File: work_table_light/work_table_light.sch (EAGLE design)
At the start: 38 parts, among them IC1 TINY24/44/84-PU, Q1 IRFP250, Q2 IRFP250, Q3 IRFP250, Q4 IRFP250, Q6 IRFP250, Q7 IRFP250

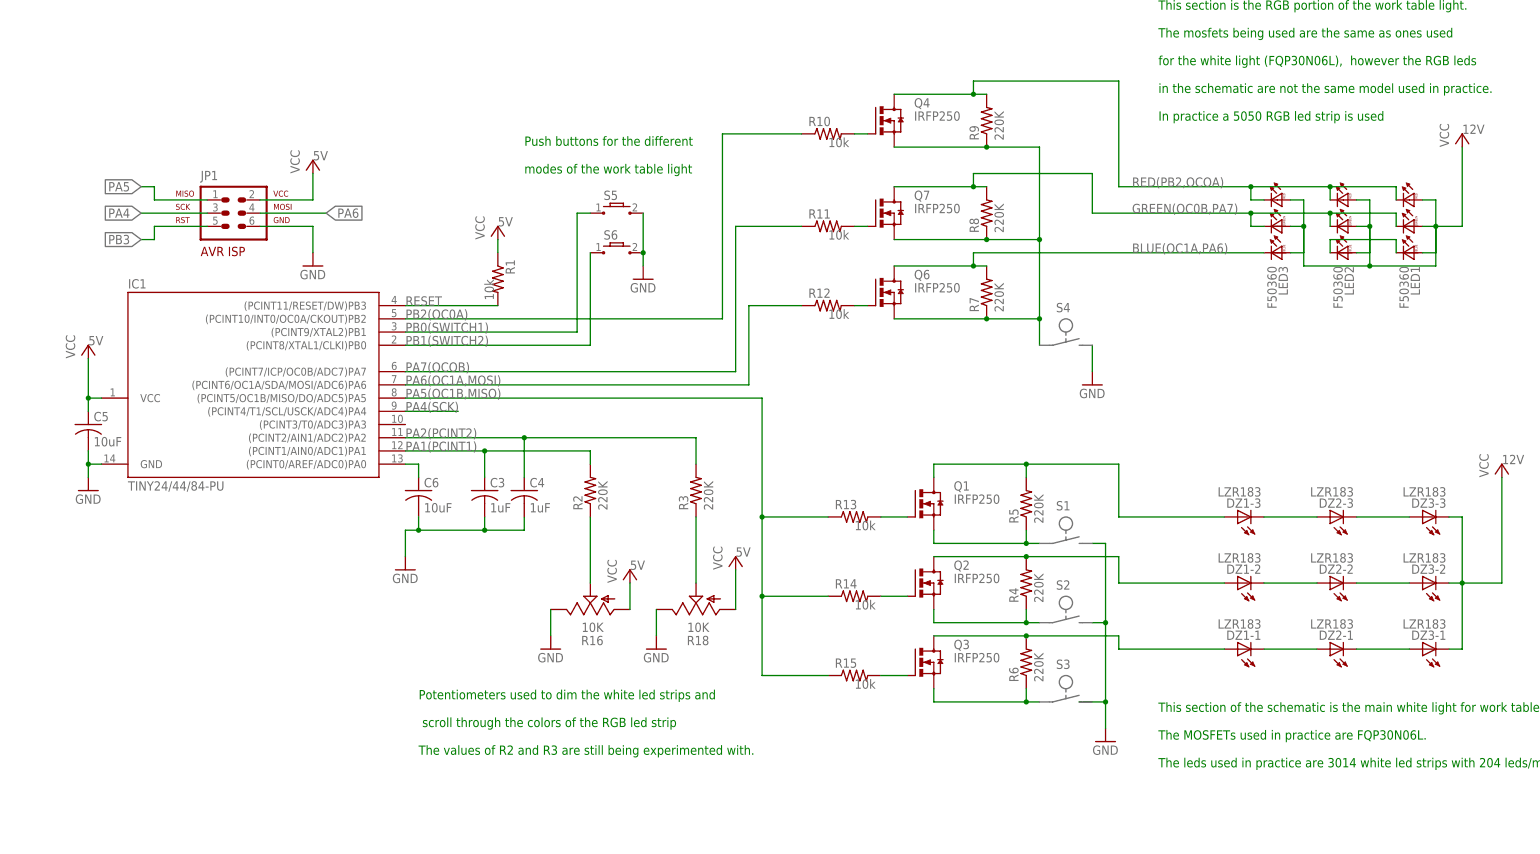
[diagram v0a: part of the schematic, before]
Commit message: updated schematic
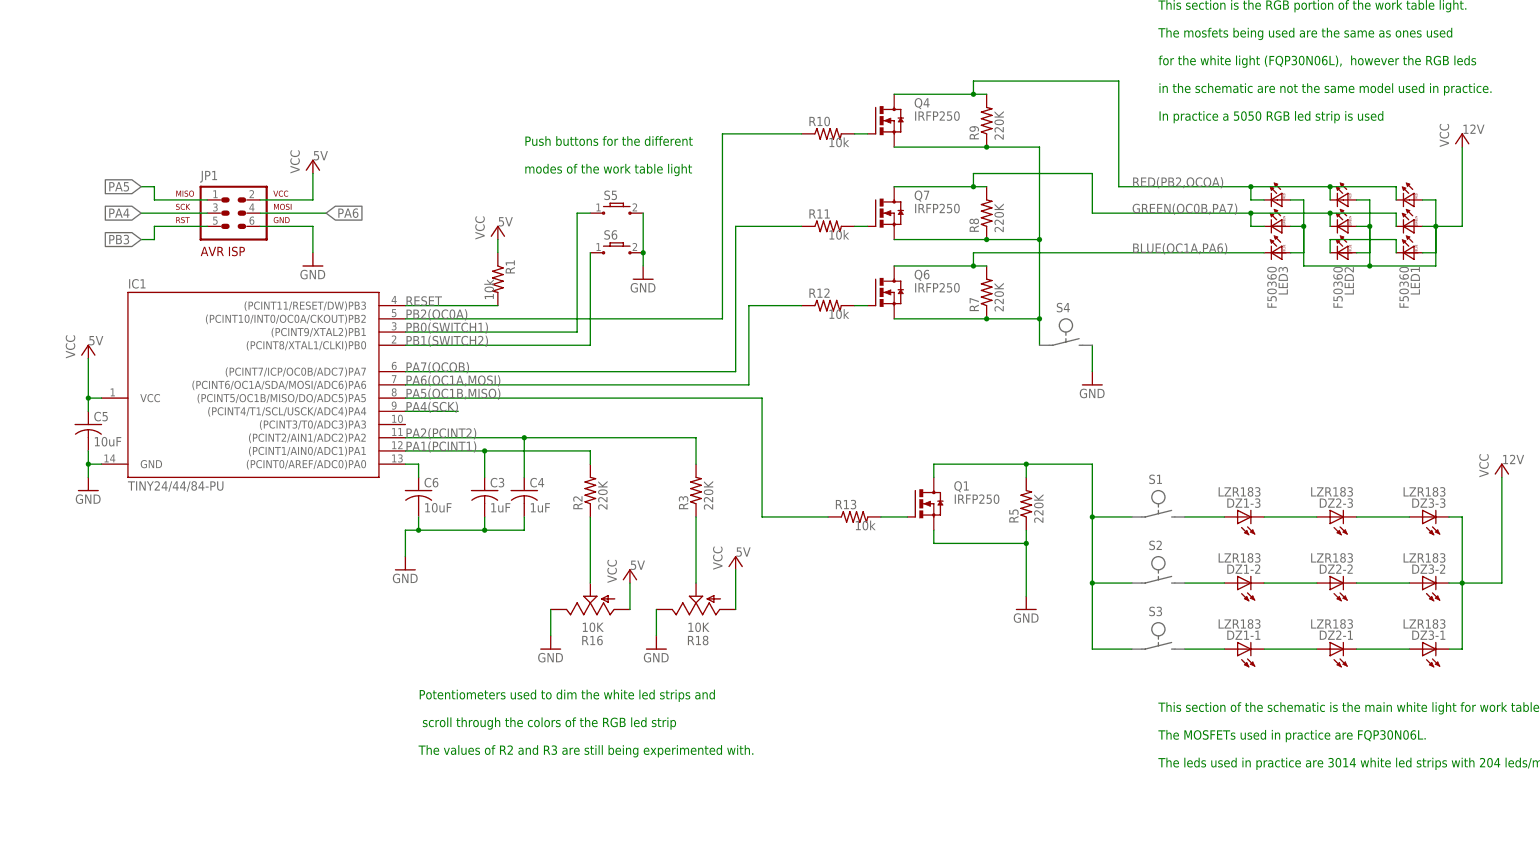
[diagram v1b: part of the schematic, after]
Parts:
- removed Q2, Q3: IRFP250, transistor-power:IRFP250
- removed R14, R15: (no value), rcl:R-US_0204/5
- removed R4, R6: 220K, resistor:R-US_0207/10
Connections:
- removed net N$14: DZ1-2.A, Q2.D, R4.2
- removed net N$17: DZ1-3.A, Q1.D, R5.2
- removed net N$20: Q3.G, R15.2
- removed net N$9: Q2.G, R14.2
- net GND: now also Q1.S, R5.1
- net N$11: now also Q1.D, R5.2; no longer DZ1-1.A, Q3.D, R6.2
- net N$2: now also DZ1-3.A; no longer Q1.S, R5.1
- net N$4: now also DZ1-2.A; no longer Q2.S, R4.1
- net N$5: now also DZ1-1.A; no longer Q3.S, R6.1
- net PA5(OC1B,MISO): no longer R14.1, R15.1
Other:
- moved on the sheet: S1, S2, S3
